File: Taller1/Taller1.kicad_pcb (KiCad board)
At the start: 2 copper layers, 85.7 x 137.2 mm, 9 parts, among them U1 DHT11, U4 SX1262-XIAO

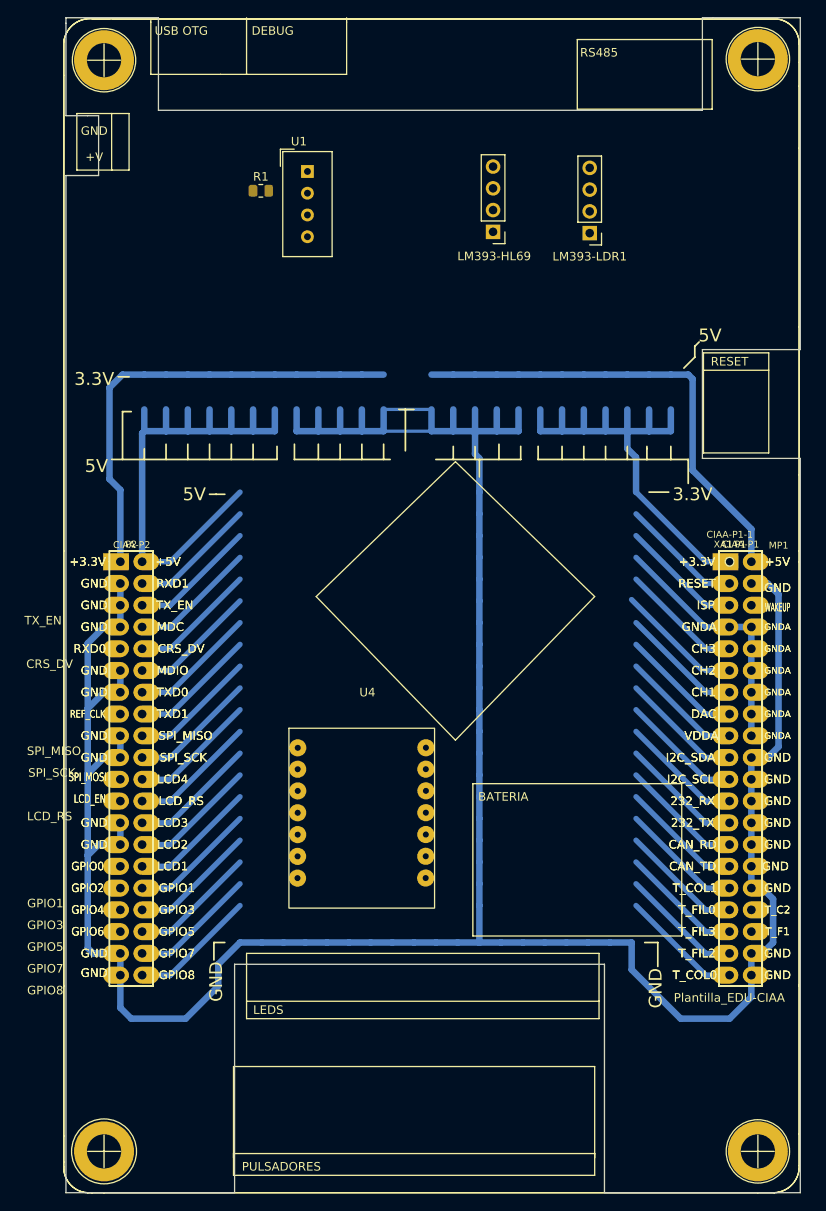
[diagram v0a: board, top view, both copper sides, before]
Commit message: ultima version PCB
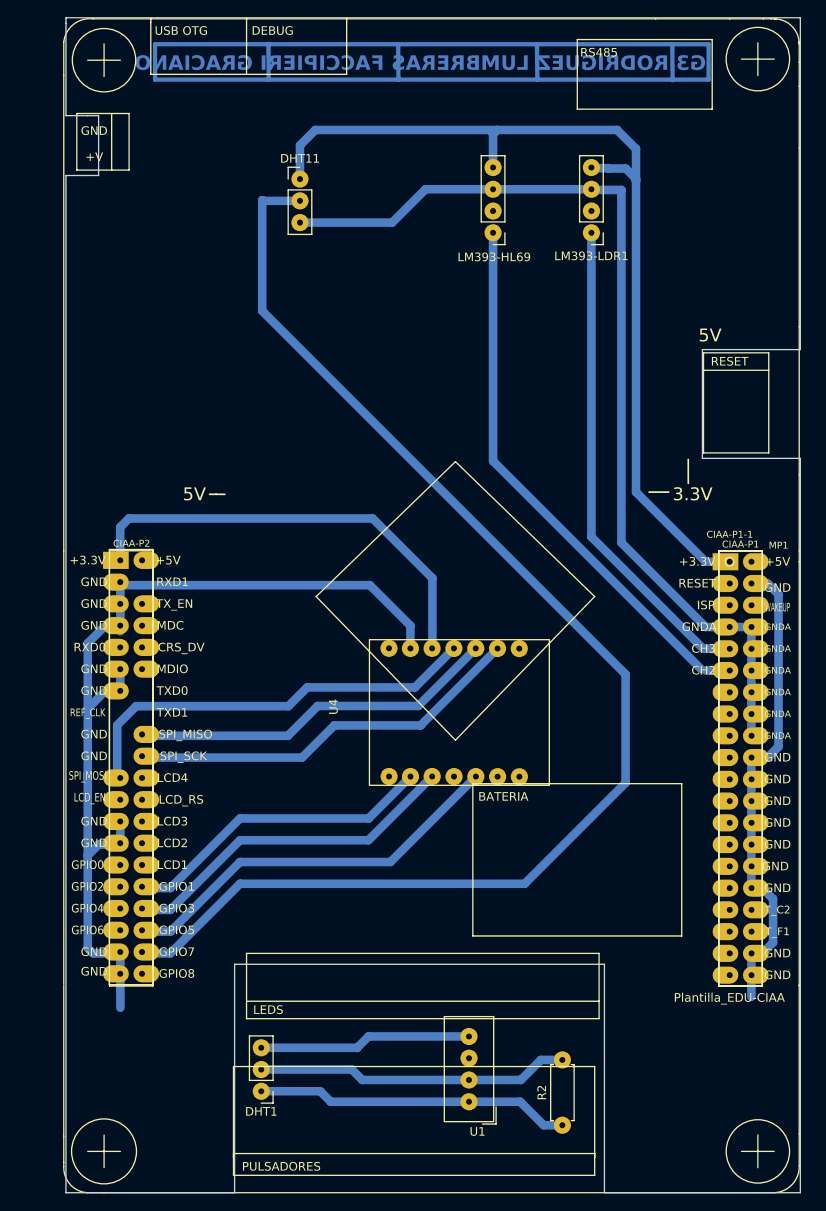
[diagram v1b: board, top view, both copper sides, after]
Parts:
- removed R1: 4,7k, Resistor_SMD:R_0805_2012Metric
- removed XA1: , mod:poncho_grande
- added DHT1: Conn_01x03, Connector_PinHeader_2.54mm:PinHeader_1x03_P2.54mm_Vertical, F.Cu at (96.5, 150.7)
- added DHT11: Conn_01x03, Connector_PinHeader_2.54mm:PinHeader_1x03_P2.54mm_Vertical, F.Cu at (101.0, 44.2)
- added R2: 4700, Resistor_THT:R_Axial_DIN0207_L6.3mm_D2.5mm_P7.62mm_Horizontal, F.Cu at (131.6, 154.7)
- moved U1 110.2 mm to (120.7, 151.9), turned to 180 degrees
- moved U4 12.1 mm to (99.2, 106.0), turned to 90 degrees
- moved LM393-LDR1 0.20 mm to (135.0, 50.5)
- moved CIAA-P2-1 0.16 mm to (81.5, 88.1)
- moved LM393-HL69 0.11 mm to (123.5, 50.5)
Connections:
- CIAA-P1-1 pad 7: unconnected-(CIAA-P1-1-GNDA-Pad7) -> GNDA
- CIAA-P2-1 pad 29: GPIO0 -> unconnected-(CIAA-P2-1-GPIO0-Pad29)
- CIAA-P2-1 pad 31: GPIO2 -> unconnected-(CIAA-P2-1-GPIO2-Pad31)
- CIAA-P2-1 pad 36: unconnected-(CIAA-P2-1-GPIO5-Pad36) -> GPIO5
- CIAA-P2-1 pad 38: unconnected-(CIAA-P2-1-GPIO7-Pad38) -> GPIO7
- U1 pad 1: Alimentacion 3.3v -> Net-(U1-VDD)
- U1 pad 4: GND -> unconnected-(U1-GND-Pad4)
- U4 pad 10: GPIO1 -> GPIO3
- U4 pad 12: GPIO2 -> GPIO5
- U4 pad 9: GPIO3 -> GPIO1
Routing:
- net GPIO7: track 0.00 -> 154.7 mm
- net GND: track 336.4 -> 200.7 mm
- net unconnected-(CIAA-P1-1-3V3-Pad1): track 0.00 -> 109.7 mm
- net (no net): track 0.00 -> 76.0 mm
- net +5VP: track 64.0 -> 0.00 mm
- net ADC2: track 0.00 -> 63.9 mm
- net ADC3: track 0.00 -> 57.0 mm
- net +5V: track 55.4 -> 0.00 mm
- net +3.3V: track 54.8 -> 0.00 mm
- net +3.3VP: track 54.0 -> 0.00 mm
- net Alimentacion 3.3v: track 0.00 -> 52.0 mm
- net SPI/MOSI: track 0.00 -> 49.9 mm
- net SPI/SCK: track 0.00 -> 46.8 mm
- net GPIO5: track 0.00 -> 46.5 mm
- net SPI/MISO: track 0.00 -> 43.2 mm
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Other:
- outline, holes or cut-outs redrawn
- board text added: "G3 RODRIGUEZ LUMBRERAS FACCIPIERI GRACIANO"
- board text removed: "CRS_DV"
- board text removed: "GND"
- board text removed: "GPIO1"
- board text removed: "GPIO3"
- board text removed: "GPIO5"
- board text removed: "GPIO7"
- board text removed: "GPIO8"
- board text removed: "LCD_RS"
- board text removed: "SPI_MISO"
- board text removed: "SPI_SCK"
- board text removed: "TX_EN"
